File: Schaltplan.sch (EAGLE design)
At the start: 14 parts, among them IC1 ICL7665CSA, Q2 IRF4905

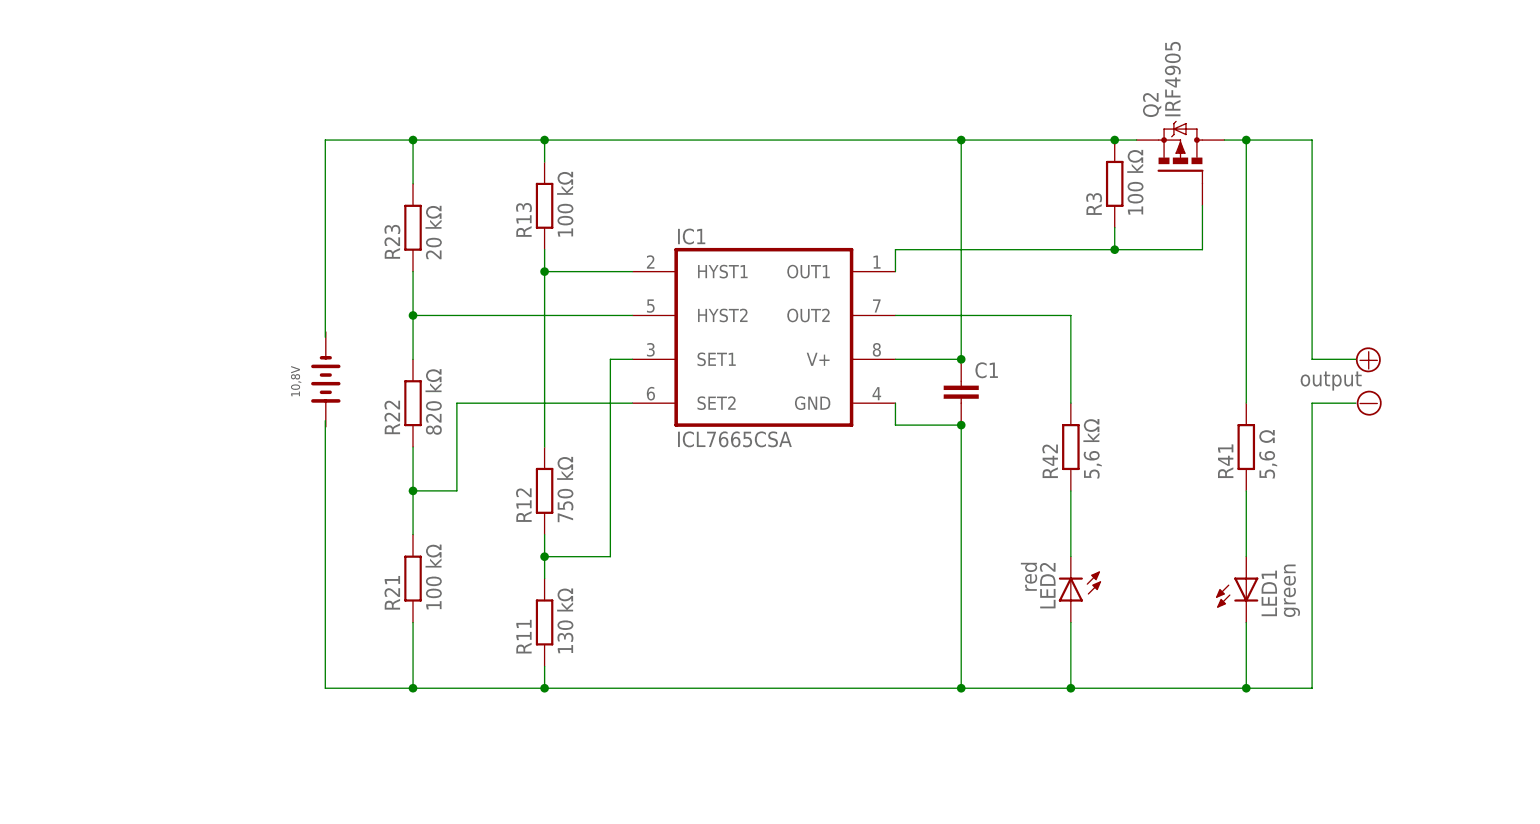
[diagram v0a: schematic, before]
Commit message: v 1.2
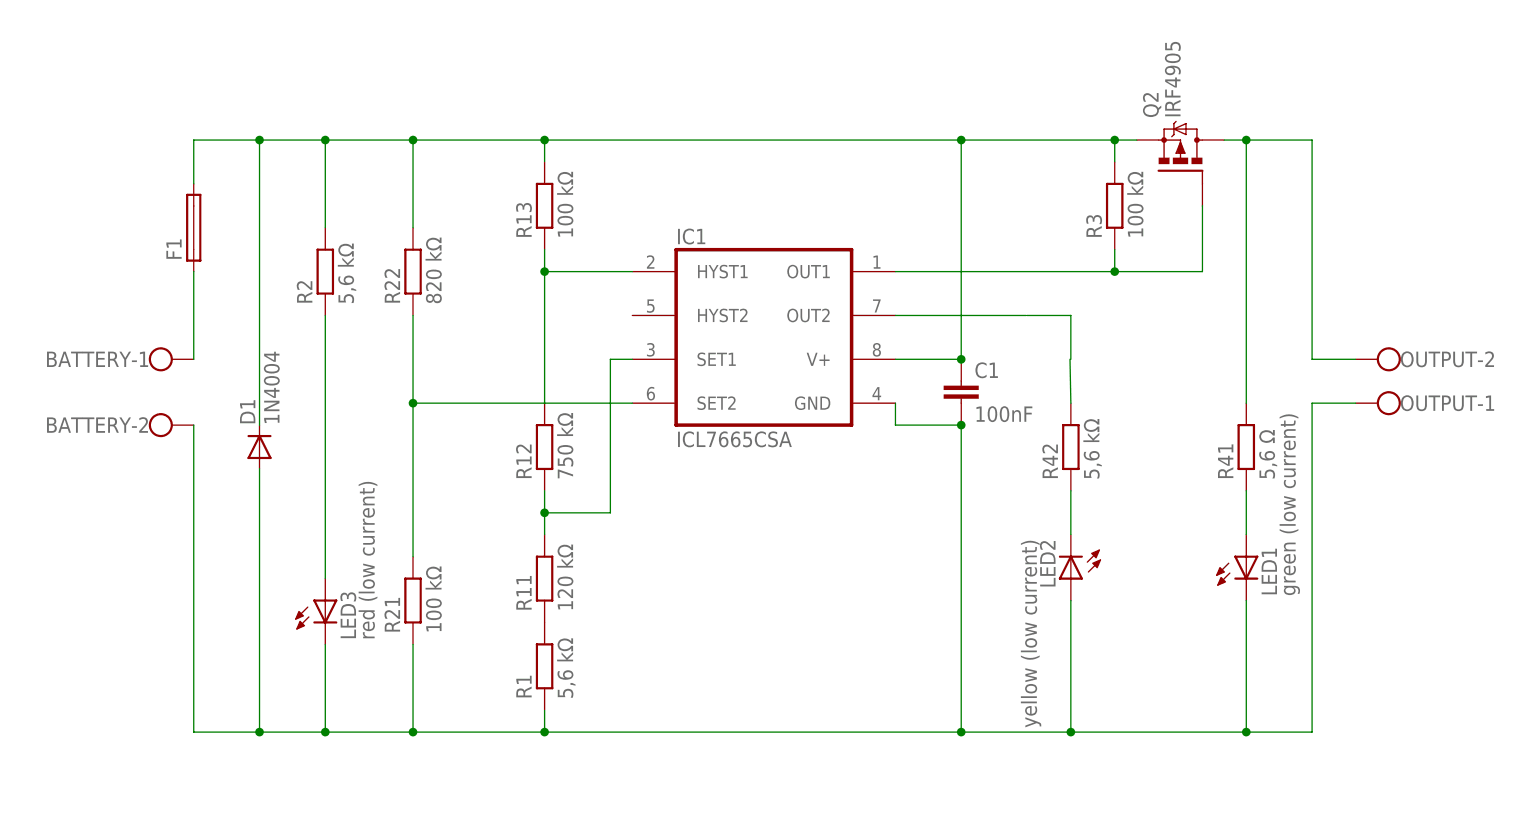
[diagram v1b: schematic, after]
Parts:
- removed R23: 20 kΩ, eagle-ltspice:RR1206
- added BATTERY, OUTPUT: (no value), con-wago-500:W237-102
- added D1: 1N4004, diode:1N4004
- added F1: (no value), fuse:GSH15
- added LED3: red (low current), led:LEDKA-3528ASYC
- added R1, R2: 5,6 kΩ, eagle-ltspice:RR1206
- C1: value (none) -> 100nF
- LED1: value green -> green (low current)
- LED2: value red -> yellow (low current); device led:LEDSML0603 -> led:LEDKA-3528ASYC
- R11: value 130 kΩ -> 120 kΩ
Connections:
- removed net OUT-POWER: Q2.D, R41.2
- new net N$10: R42.2
- new net N$17: R1.2, R11.1
- new net N$18: BATTERY-1.KL, F1.1
- new net N$4: OUTPUT-2.KL, Q2.D, R41.2
- net GND: now also BATTERY-2.KL, D1.A, LED3.C, OUTPUT-1.KL, R1.1; no longer R11.1
- net N$1: now also LED3.A, R2.1; no longer IC1.HYST2, R22.2, R23.1
- net N$5: no longer R42.2
- net POWER: now also D1.C, F1.2, R2.2, R22.2; no longer R23.2
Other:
- note removed: "10,8V"
- note removed: "output"
- moved on the sheet: LED1, LED2, R11, R12, R21, R22, R3
